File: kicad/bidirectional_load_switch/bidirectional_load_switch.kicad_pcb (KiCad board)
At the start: 2 copper layers, 0 parts

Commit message: load switch
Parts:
- added C101: 100n, Capacitor_SMD:C_0603_1608Metric, F.Cu at (133.9, 45.6)
- added C102: 10u, Capacitor_SMD:C_1206_3216Metric, F.Cu at (136.1, 45.6)
- added C103: 10u, Capacitor_SMD:C_1206_3216Metric, F.Cu at (127.0, 45.6)
- added C104: 100n, Capacitor_SMD:C_0603_1608Metric, F.Cu at (129.2, 45.6)
- added C201: 1u, Capacitor_SMD:C_0603_1608Metric, F.Cu at (126.4, 51.0)
- added C202: 100n, Capacitor_SMD:C_0603_1608Metric, F.Cu at (128.2, 51.0)
- added C203: 10u, Capacitor_SMD:C_1206_3216Metric, F.Cu at (150.1, 46.0)
- added C204: 100n, Capacitor_SMD:C_0603_1608Metric, F.Cu at (149.8, 48.0)
- added C301: 1u, Capacitor_SMD:C_0603_1608Metric, F.Cu at (126.4, 65.5)
- added C302: 100n, Capacitor_SMD:C_0603_1608Metric, F.Cu at (128.2, 65.5)
- added C303: 10u, Capacitor_SMD:C_1206_3216Metric, F.Cu at (150.1, 60.5)
- added C304: 100n, Capacitor_SMD:C_0603_1608Metric, F.Cu at (149.8, 62.5)
- added C401: 1u, Capacitor_SMD:C_0603_1608Metric, F.Cu at (126.4, 80.0)
- added C402: 100n, Capacitor_SMD:C_0603_1608Metric, F.Cu at (128.2, 80.0)
- added C403: 10u, Capacitor_SMD:C_1206_3216Metric, F.Cu at (150.1, 75.0)
- added C404: 100n, Capacitor_SMD:C_0603_1608Metric, F.Cu at (149.8, 77.0)
- added C501: 1u, Capacitor_SMD:C_0603_1608Metric, F.Cu at (126.4, 94.5)
- added C502: 100n, Capacitor_SMD:C_0603_1608Metric, F.Cu at (128.2, 94.5)
- added C503: 10u, Capacitor_SMD:C_1206_3216Metric, F.Cu at (150.1, 89.5)
- added C504: 100n, Capacitor_SMD:C_0603_1608Metric, F.Cu at (149.8, 91.5)
- added C601: 1u, Capacitor_SMD:C_0603_1608Metric, F.Cu at (126.4, 109.0)
- added C602: 100n, Capacitor_SMD:C_0603_1608Metric, F.Cu at (128.2, 109.0)
- added C603: 10u, Capacitor_SMD:C_1206_3216Metric, F.Cu at (150.1, 104.0)
- added C604: 100n, Capacitor_SMD:C_0603_1608Metric, F.Cu at (149.8, 106.0)
- added C701: 1u, Capacitor_SMD:C_0603_1608Metric, F.Cu at (126.4, 123.5)
- added C702: 100n, Capacitor_SMD:C_0603_1608Metric, F.Cu at (128.2, 123.5)
- added C703: 10u, Capacitor_SMD:C_1206_3216Metric, F.Cu at (150.1, 118.5)
- added C704: 100n, Capacitor_SMD:C_0603_1608Metric, F.Cu at (149.8, 120.5)
- added C801: 1u, Capacitor_SMD:C_0603_1608Metric, F.Cu at (126.4, 137.9)
- added C802: 100n, Capacitor_SMD:C_0603_1608Metric, F.Cu at (128.2, 137.9)
- added C803: 10u, Capacitor_SMD:C_1206_3216Metric, F.Cu at (150.1, 133.1)
- added C804: 100n, Capacitor_SMD:C_0603_1608Metric, F.Cu at (149.8, 135.1)
- added C901: 1u, Capacitor_SMD:C_0603_1608Metric, F.Cu at (126.4, 152.4)
- added C902: 100n, Capacitor_SMD:C_0603_1608Metric, F.Cu at (128.2, 152.4)
- added C903: 10u, Capacitor_SMD:C_1206_3216Metric, F.Cu at (150.1, 147.6)
- added C904: 100n, Capacitor_SMD:C_0603_1608Metric, F.Cu at (149.8, 149.6)
- added J101: 282838-2, screw_terminal_282838-2:CONN2_282838-2_TEC, F.Cu at (168.6, 38.1)
- added J102: Conn_01x02_Socket, Connector_PinHeader_2.54mm:PinHeader_1x02_P2.54mm_Vertical, F.Cu at (148.3, 41.1)
- added J103: Conn_01x09_Socket, Connector_PinHeader_2.54mm:PinHeader_1x09_P2.54mm_Vertical, F.Cu at (120.3, 41.1)
- added J104: Conn_01x02_Socket, Connector_PinHeader_2.54mm:PinHeader_1x02_P2.54mm_Vertical, F.Cu at (133.3, 41.1)
- added LED201: B1911PG--20D000514U1930, led_B1911PG--20D000514U1930:LED_B1911PG--20D000514U1930_HVK, F.Cu at (128.8, 54.9)
- added LED301: B1911PG--20D000514U1930, led_B1911PG--20D000514U1930:LED_B1911PG--20D000514U1930_HVK, F.Cu at (128.9, 69.3)
- added LED401: B1911PG--20D000514U1930, led_B1911PG--20D000514U1930:LED_B1911PG--20D000514U1930_HVK, F.Cu at (128.8, 83.8)
- added LED501: B1911PG--20D000514U1930, led_B1911PG--20D000514U1930:LED_B1911PG--20D000514U1930_HVK, F.Cu at (128.8, 98.3)
- added LED601: B1911PG--20D000514U1930, led_B1911PG--20D000514U1930:LED_B1911PG--20D000514U1930_HVK, F.Cu at (128.8, 112.8)
- added LED701: B1911PG--20D000514U1930, led_B1911PG--20D000514U1930:LED_B1911PG--20D000514U1930_HVK, F.Cu at (128.8, 127.3)
- added LED801: B1911PG--20D000514U1930, led_B1911PG--20D000514U1930:LED_B1911PG--20D000514U1930_HVK, F.Cu at (128.8, 141.8)
- added LED901: B1911PG--20D000514U1930, led_B1911PG--20D000514U1930:LED_B1911PG--20D000514U1930_HVK, F.Cu at (128.8, 156.3)
- added R201: 150, Resistor_SMD:R_0603_1608Metric, F.Cu at (131.8, 54.9)
- added R202: 50, Resistor_SMD:R_0603_1608Metric, F.Cu at (133.8, 49.9)
- added R203: 50, Resistor_SMD:R_0603_1608Metric, F.Cu at (133.8, 52.1)
- added R204: 5, Resistor_SMD:R_0805_2012Metric, F.Cu at (152.1, 50.0)
- added R205: 5, Resistor_SMD:R_0805_2012Metric, F.Cu at (152.1, 52.0)
- added R301: 150, Resistor_SMD:R_0603_1608Metric, F.Cu at (131.8, 69.3)
- added R302: 50, Resistor_SMD:R_0603_1608Metric, F.Cu at (133.8, 64.4)
- added R303: 50, Resistor_SMD:R_0603_1608Metric, F.Cu at (133.8, 66.6)
- added R304: 5, Resistor_SMD:R_0805_2012Metric, F.Cu at (152.1, 64.5)
- added R305: 5, Resistor_SMD:R_0805_2012Metric, F.Cu at (152.1, 66.5)
- added R401: 150, Resistor_SMD:R_0603_1608Metric, F.Cu at (131.8, 83.8)
- added R402: 50, Resistor_SMD:R_0603_1608Metric, F.Cu at (133.8, 78.9)
- added R403: 50, Resistor_SMD:R_0603_1608Metric, F.Cu at (133.8, 81.1)
- added R404: 5, Resistor_SMD:R_0805_2012Metric, F.Cu at (152.1, 79.0)
- added R405: 5, Resistor_SMD:R_0805_2012Metric, F.Cu at (152.1, 81.0)
- added R501: 150, Resistor_SMD:R_0603_1608Metric, F.Cu at (131.8, 98.3)
- added R502: 50, Resistor_SMD:R_0603_1608Metric, F.Cu at (133.8, 93.4)
- added R503: 50, Resistor_SMD:R_0603_1608Metric, F.Cu at (133.8, 95.6)
- added R504: 5, Resistor_SMD:R_0805_2012Metric, F.Cu at (152.1, 93.5)
- added R505: 5, Resistor_SMD:R_0805_2012Metric, F.Cu at (152.1, 95.5)
- added R601: 150, Resistor_SMD:R_0603_1608Metric, F.Cu at (131.8, 112.8)
- added R602: 50, Resistor_SMD:R_0603_1608Metric, F.Cu at (133.8, 107.9)
- added R603: 50, Resistor_SMD:R_0603_1608Metric, F.Cu at (133.8, 110.1)
- added R604: 5, Resistor_SMD:R_0805_2012Metric, F.Cu at (152.1, 108.0)
- added R605: 5, Resistor_SMD:R_0805_2012Metric, F.Cu at (152.1, 110.0)
- added R701: 150, Resistor_SMD:R_0603_1608Metric, F.Cu at (131.8, 127.3)
- added R702: 50, Resistor_SMD:R_0603_1608Metric, F.Cu at (133.8, 122.4)
- added R703: 50, Resistor_SMD:R_0603_1608Metric, F.Cu at (133.8, 124.6)
- added R704: 5, Resistor_SMD:R_0805_2012Metric, F.Cu at (152.1, 122.5)
- added R705: 5, Resistor_SMD:R_0805_2012Metric, F.Cu at (152.1, 124.5)
- added R801: 150, Resistor_SMD:R_0603_1608Metric, F.Cu at (131.8, 141.8)
- added R802: 50, Resistor_SMD:R_0603_1608Metric, F.Cu at (133.8, 136.9)
- added R803: 50, Resistor_SMD:R_0603_1608Metric, F.Cu at (133.8, 139.1)
- added R804: 5, Resistor_SMD:R_0805_2012Metric, F.Cu at (152.1, 137.1)
- added R805: 5, Resistor_SMD:R_0805_2012Metric, F.Cu at (152.1, 139.1)
- added R901: 150, Resistor_SMD:R_0603_1608Metric, F.Cu at (131.8, 156.3)
- added R902: 50, Resistor_SMD:R_0603_1608Metric, F.Cu at (133.8, 151.4)
- added R903: 50, Resistor_SMD:R_0603_1608Metric, F.Cu at (133.8, 153.6)
- added R904: 5, Resistor_SMD:R_0805_2012Metric, F.Cu at (152.1, 151.6)
- added R905: 5, Resistor_SMD:R_0805_2012Metric, F.Cu at (152.1, 153.6)
- added RS101: R_US, Resistor_SMD:R_2512_6332Metric, F.Cu at (163.5, 48.2)
- added RS102: R_US, Resistor_SMD:R_2512_6332Metric, F.Cu at (163.6, 62.6)
- added RS103: R_US, Resistor_SMD:R_2512_6332Metric, F.Cu at (163.6, 77.2)
- added RS104: R_US, Resistor_SMD:R_2512_6332Metric, F.Cu at (163.6, 91.7)
- added RS105: R_US, Resistor_SMD:R_2512_6332Metric, F.Cu at (163.6, 106.2)
- added RS106: R_US, Resistor_SMD:R_2512_6332Metric, F.Cu at (163.6, 120.7)
- added RS107: R_US, Resistor_SMD:R_2512_6332Metric, F.Cu at (163.6, 135.2)
- added RS108: R_US, Resistor_SMD:R_2512_6332Metric, F.Cu at (163.6, 149.7)
- added U101: LDL212PV33R, ldo_LDL212PV33R:DFN_V33R_STM, F.Cu at (131.6, 45.6)
- added U201: SN74LVC1G17DCKR, buffer_SN74LVC1G17DCKR:DCK5, F.Cu at (130.6, 51.0)
- added U202: UCC23313DWYR, gate_driver_UCC23313DWYR:SOIC6_DWY_TEX, F.Cu at (142.1, 51.0)
- added U203: SISS94DN-T1-GE3, mosfet_SISS94DN-T1-GE3:MOSFET_3DN-T1-GE3_VIS, F.Cu at (156.2, 48.7)
- added U204: SISS94DN-T1-GE3, mosfet_SISS94DN-T1-GE3:MOSFET_3DN-T1-GE3_VIS, F.Cu at (156.2, 54.4)
- added U301: SN74LVC1G17DCKR, buffer_SN74LVC1G17DCKR:DCK5, F.Cu at (130.6, 65.5)
- added U302: UCC23313DWYR, gate_driver_UCC23313DWYR:SOIC6_DWY_TEX, F.Cu at (142.1, 65.5)
- added U303: SISS94DN-T1-GE3, mosfet_SISS94DN-T1-GE3:MOSFET_3DN-T1-GE3_VIS, F.Cu at (156.2, 63.2)
- added U304: SISS94DN-T1-GE3, mosfet_SISS94DN-T1-GE3:MOSFET_3DN-T1-GE3_VIS, F.Cu at (156.2, 68.9)
- added U401: SN74LVC1G17DCKR, buffer_SN74LVC1G17DCKR:DCK5, F.Cu at (130.6, 80.0)
- added U402: UCC23313DWYR, gate_driver_UCC23313DWYR:SOIC6_DWY_TEX, F.Cu at (142.1, 80.0)
- added U403: SISS94DN-T1-GE3, mosfet_SISS94DN-T1-GE3:MOSFET_3DN-T1-GE3_VIS, F.Cu at (156.2, 77.7)
- added U404: SISS94DN-T1-GE3, mosfet_SISS94DN-T1-GE3:MOSFET_3DN-T1-GE3_VIS, F.Cu at (156.2, 83.4)
- added U501: SN74LVC1G17DCKR, buffer_SN74LVC1G17DCKR:DCK5, F.Cu at (130.6, 94.5)
- added U502: UCC23313DWYR, gate_driver_UCC23313DWYR:SOIC6_DWY_TEX, F.Cu at (142.1, 94.5)
- added U503: SISS94DN-T1-GE3, mosfet_SISS94DN-T1-GE3:MOSFET_3DN-T1-GE3_VIS, F.Cu at (156.2, 92.2)
- added U504: SISS94DN-T1-GE3, mosfet_SISS94DN-T1-GE3:MOSFET_3DN-T1-GE3_VIS, F.Cu at (156.2, 97.9)
- added U601: SN74LVC1G17DCKR, buffer_SN74LVC1G17DCKR:DCK5, F.Cu at (130.6, 109.0)
- added U602: UCC23313DWYR, gate_driver_UCC23313DWYR:SOIC6_DWY_TEX, F.Cu at (142.1, 109.0)
- added U603: SISS94DN-T1-GE3, mosfet_SISS94DN-T1-GE3:MOSFET_3DN-T1-GE3_VIS, F.Cu at (156.2, 106.7)
- added U604: SISS94DN-T1-GE3, mosfet_SISS94DN-T1-GE3:MOSFET_3DN-T1-GE3_VIS, F.Cu at (156.2, 112.4)
- added U701: SN74LVC1G17DCKR, buffer_SN74LVC1G17DCKR:DCK5, F.Cu at (130.6, 123.5)
- added U702: UCC23313DWYR, gate_driver_UCC23313DWYR:SOIC6_DWY_TEX, F.Cu at (142.1, 123.5)
- added U703: SISS94DN-T1-GE3, mosfet_SISS94DN-T1-GE3:MOSFET_3DN-T1-GE3_VIS, F.Cu at (156.2, 121.2)
- added U704: SISS94DN-T1-GE3, mosfet_SISS94DN-T1-GE3:MOSFET_3DN-T1-GE3_VIS, F.Cu at (156.2, 126.9)
- added U801: SN74LVC1G17DCKR, buffer_SN74LVC1G17DCKR:DCK5, F.Cu at (130.6, 138.0)
- added U802: UCC23313DWYR, gate_driver_UCC23313DWYR:SOIC6_DWY_TEX, F.Cu at (142.1, 138.0)
- added U803: SISS94DN-T1-GE3, mosfet_SISS94DN-T1-GE3:MOSFET_3DN-T1-GE3_VIS, F.Cu at (156.2, 135.7)
- added U804: SISS94DN-T1-GE3, mosfet_SISS94DN-T1-GE3:MOSFET_3DN-T1-GE3_VIS, F.Cu at (156.2, 141.4)
- added U901: SN74LVC1G17DCKR, buffer_SN74LVC1G17DCKR:DCK5, F.Cu at (130.6, 152.5)
- added U902: UCC23313DWYR, gate_driver_UCC23313DWYR:SOIC6_DWY_TEX, F.Cu at (142.1, 152.5)
- added U903: SISS94DN-T1-GE3, mosfet_SISS94DN-T1-GE3:MOSFET_3DN-T1-GE3_VIS, F.Cu at (156.2, 150.2)
- added U904: SISS94DN-T1-GE3, mosfet_SISS94DN-T1-GE3:MOSFET_3DN-T1-GE3_VIS, F.Cu at (156.2, 155.9)
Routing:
- net 3V3: track 0.00 -> 209.9 mm
- net /PWM8: track 0.00 -> 106.1 mm
- net /PWM7: track 0.00 -> 94.1 mm
- net /PWM6: track 0.00 -> 82.1 mm
- net /PWM5: track 0.00 -> 70.1 mm
- net /PWM4: track 0.00 -> 58.2 mm
- net /PWM3: track 0.00 -> 46.1 mm
- net /PWM2: track 0.00 -> 34.2 mm
- net /PWM1: track 0.00 -> 22.3 mm
- net GND: track 0.00 -> 10.5 mm, vias 0 -> 78
- net Net-(U902-CATHODE): track 0.00 -> 2.15 mm
- net Net-(U802-CATHODE): track 0.00 -> 2.15 mm
- net Net-(U702-CATHODE): track 0.00 -> 2.15 mm
- net Net-(U602-CATHODE): track 0.00 -> 2.15 mm
- net Net-(U502-CATHODE): track 0.00 -> 2.15 mm
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- added copper zone on F.Cu, net /AC_in
- added copper zone on F.Cu, net /Channel 1/RIN
- added copper zone on F.Cu, net /Channel 2/RIN
- added copper zone on F.Cu, net /Channel 3/RIN
- added copper zone on F.Cu, net /Channel 4/RIN
- added copper zone on F.Cu, net /Channel 5/RIN
- added copper zone on F.Cu, net /Channel 6/RIN
- added copper zone on F.Cu, net /Channel 7/RIN
- added copper zone on F.Cu, net /Channel 8/RIN
- added copper zone on B.Cu, net 15V_isolated
- added copper zone on F.Cu, net 15V_isolated
- added copper zone on F.Cu, net 3V3
- added copper zone on F.Cu, net 5V
- added copper zone on B.Cu, net Earth
- added copper zone on F.Cu, net Earth
- added copper zone on B.Cu, net GND
- added copper zone on F.Cu, net GND
- added copper zone on B.Cu, net GNDPWR
- added copper zone on F.Cu, net GNDPWR
- added copper zone on F.Cu, net Net-(U202-VOUT)
- added copper zone on F.Cu, net Net-(U203-G)
- added copper zone on F.Cu, net Net-(U204-G)
- added copper zone on F.Cu, net Net-(U302-VOUT)
- added copper zone on F.Cu, net Net-(U303-G)
- added copper zone on F.Cu, net Net-(U304-G)
- added copper zone on F.Cu, net Net-(U402-VOUT)
- added copper zone on F.Cu, net Net-(U403-G)
- added copper zone on F.Cu, net Net-(U404-G)
- added copper zone on F.Cu, net Net-(U502-VOUT)
- added copper zone on F.Cu, net Net-(U503-G)
- added copper zone on F.Cu, net Net-(U504-G)
- added copper zone on F.Cu, net Net-(U602-VOUT)
- added copper zone on F.Cu, net Net-(U603-G)
- added copper zone on F.Cu, net Net-(U604-G)
- added copper zone on F.Cu, net Net-(U702-VOUT)
- added copper zone on F.Cu, net Net-(U703-G)
- added copper zone on F.Cu, net Net-(U704-G)
- added copper zone on F.Cu, net Net-(U802-VOUT)
- added copper zone on F.Cu, net Net-(U803-G)
- added copper zone on F.Cu, net Net-(U804-G)
- added copper zone on F.Cu, net Net-(U902-VOUT)
- added copper zone on F.Cu, net Net-(U903-G)
- added copper zone on F.Cu, net Net-(U904-G)
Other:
- board outline added: 54.7 x 125.5 mm

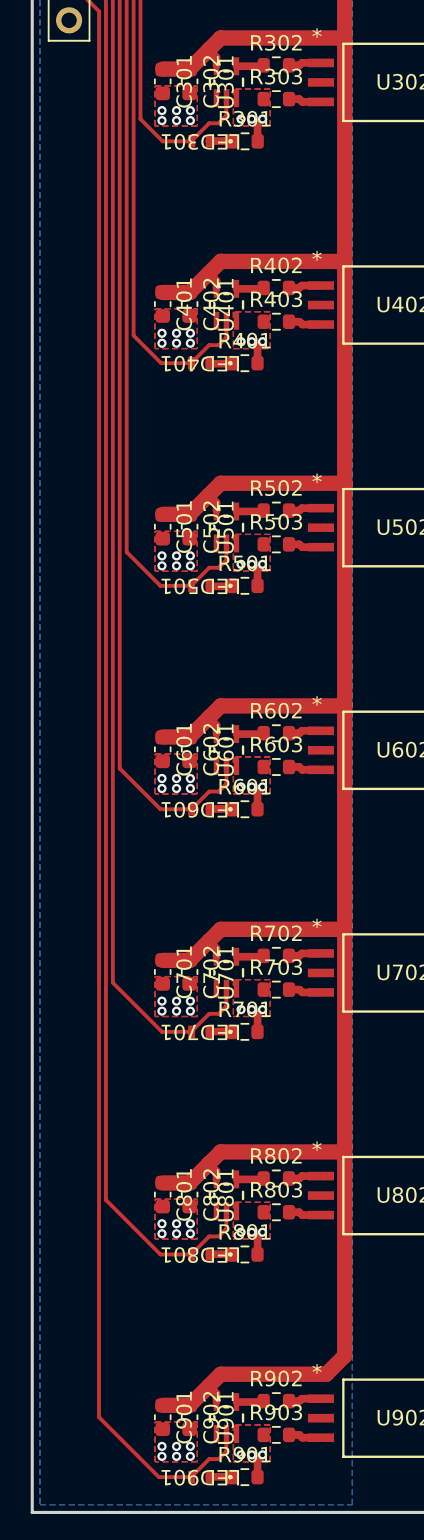
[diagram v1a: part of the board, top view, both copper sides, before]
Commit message: kicad
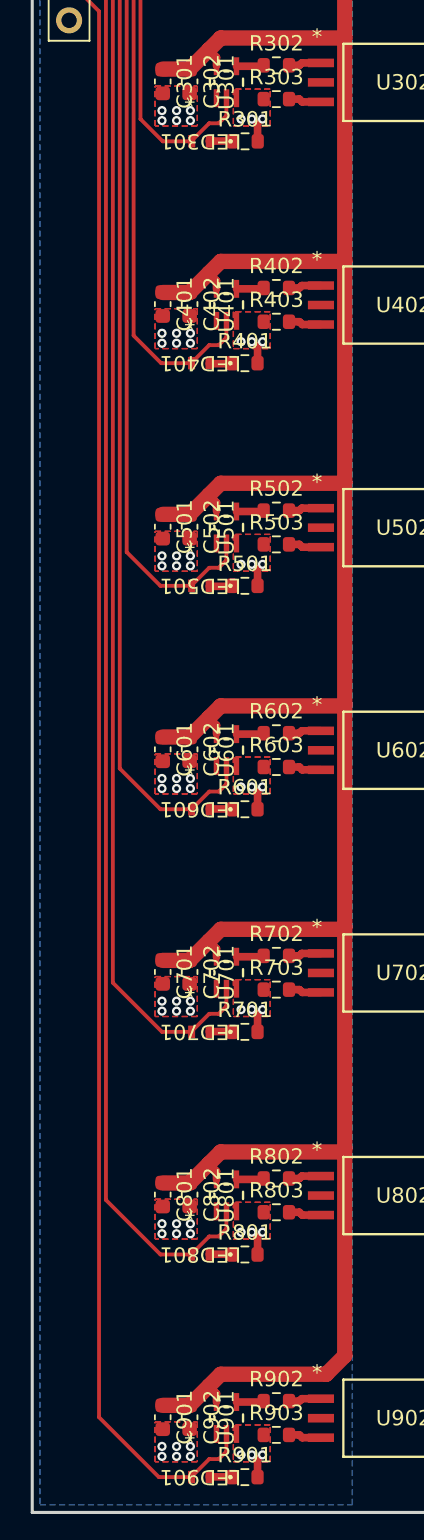
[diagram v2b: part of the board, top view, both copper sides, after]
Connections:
- net Net-(U201-Y) renamed /Channel 1/BOUT
- net Net-(U202-ANODE) renamed /Channel 1/ANODE
- net Net-(U202-VOUT) renamed /Channel 1/VOUT
- net Net-(U203-G) renamed /Channel 1/VG1
- net Net-(U204-G) renamed /Channel 1/VG2
- net Net-(U301-Y) renamed /Channel 2/BOUT
- net Net-(U302-ANODE) renamed /Channel 2/ANODE
- net Net-(U302-VOUT) renamed /Channel 2/VOUT
- net Net-(U303-G) renamed /Channel 2/VG1
- net Net-(U304-G) renamed /Channel 2/VG2
- net Net-(U401-Y) renamed /Channel 3/BOUT
- net Net-(U402-ANODE) renamed /Channel 3/ANODE
- net Net-(U402-VOUT) renamed /Channel 3/VOUT
- net Net-(U403-G) renamed /Channel 3/VG1
- net Net-(U404-G) renamed /Channel 3/VG2
- net Net-(U501-Y) renamed /Channel 4/BOUT
- net Net-(U502-ANODE) renamed /Channel 4/ANODE
- net Net-(U502-VOUT) renamed /Channel 4/VOUT
- net Net-(U503-G) renamed /Channel 4/VG1
- net Net-(U504-G) renamed /Channel 4/VG2
- net Net-(U601-Y) renamed /Channel 5/BOUT
- net Net-(U602-ANODE) renamed /Channel 5/ANODE
- net Net-(U602-VOUT) renamed /Channel 5/VOUT
- net Net-(U603-G) renamed /Channel 5/VG1
- net Net-(U604-G) renamed /Channel 5/VG2
- net Net-(U701-Y) renamed /Channel 6/BOUT
- net Net-(U702-ANODE) renamed /Channel 6/ANODE
- net Net-(U702-VOUT) renamed /Channel 6/VOUT
- net Net-(U703-G) renamed /Channel 6/VG1
- net Net-(U704-G) renamed /Channel 6/VG2
- net Net-(U801-Y) renamed /Channel 7/BOUT
- net Net-(U802-ANODE) renamed /Channel 7/ANODE
- net Net-(U802-VOUT) renamed /Channel 7/VOUT
- net Net-(U803-G) renamed /Channel 7/VG1
- net Net-(U804-G) renamed /Channel 7/VG2
- net Net-(U901-Y) renamed /Channel 8/BOUT
- net Net-(U902-ANODE) renamed /Channel 8/ANODE
- net Net-(U902-VOUT) renamed /Channel 8/VOUT
- net Net-(U903-G) renamed /Channel 8/VG1
- net Net-(U904-G) renamed /Channel 8/VG2

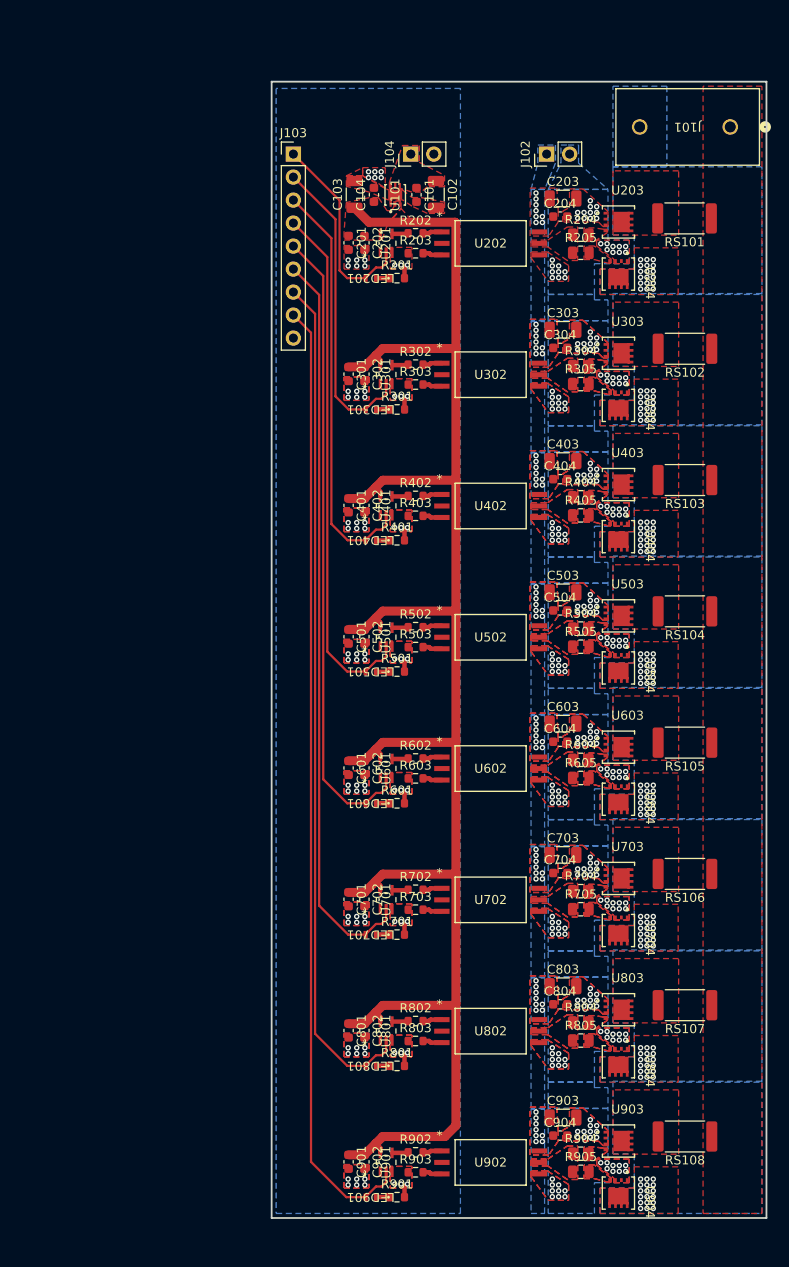
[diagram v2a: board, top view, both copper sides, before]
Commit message: kicad
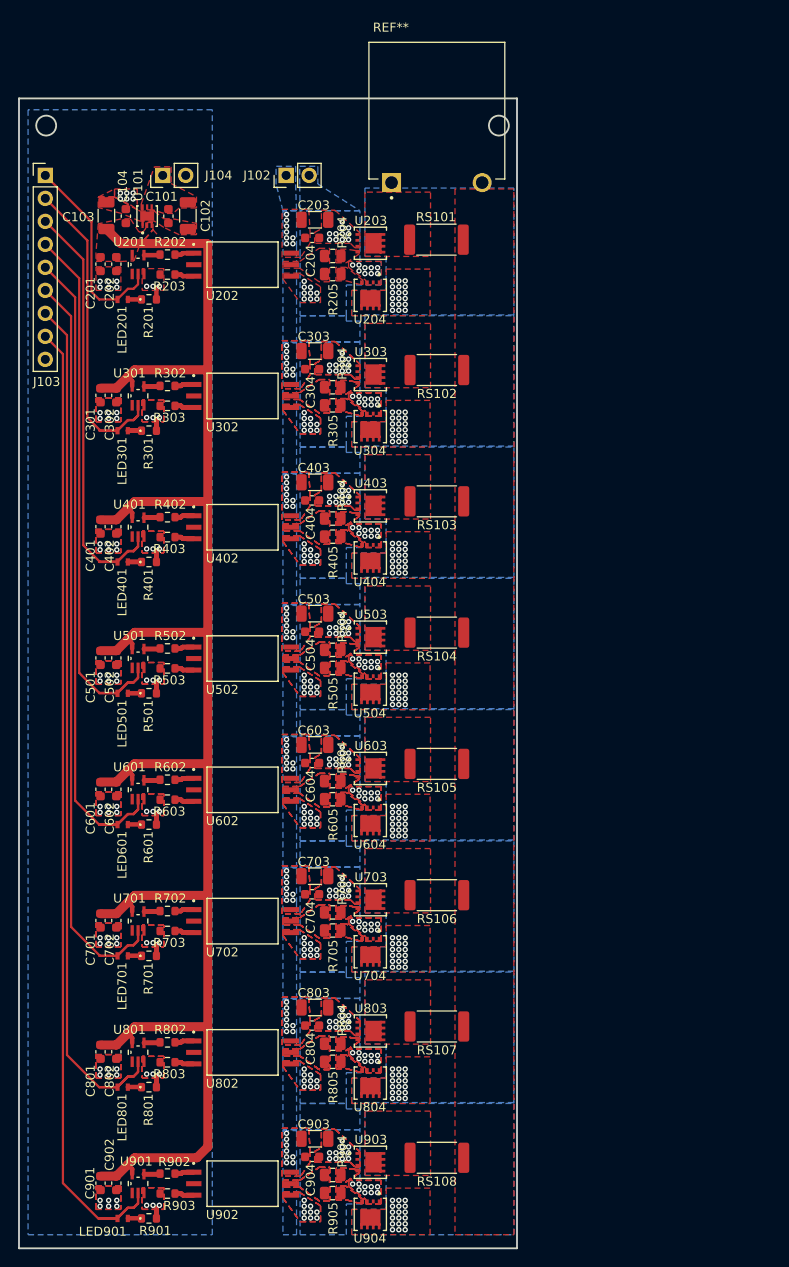
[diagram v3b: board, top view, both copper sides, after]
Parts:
- removed J101: 282838-2, screw_terminal_282838-2:CONN2_282838-2_TEC
- added REF**: TE_282852-2, screw_terminal_282852-2:TE_282852-2, F.Cu at (136.2, 44.3)
- RS101: value R_US -> 1
- RS102: value R_US -> 3.9
- RS103: value R_US -> 15
- RS104: value R_US -> 47
- RS105: value R_US -> 200
- RS106: value R_US -> 680
- RS107: value R_US -> 2700
- RS108: value R_US -> 10000
- moved J102 28.9 mm to (119.5, 43.5)
- moved R301 27.5 mm to (104.3, 71.7)
- moved LED301 27.5 mm to (101.5, 71.7)
- moved R401 27.5 mm to (104.3, 86.2)
- moved R501 27.5 mm to (104.3, 100.7)
- moved LED501 27.5 mm to (101.5, 100.7)
- moved LED401 27.5 mm to (101.5, 86.2)
- moved C101 27.5 mm to (106.5, 48.0)
- moved C102 27.5 mm to (108.7, 48.0)
- moved C201 27.5 mm to (99.0, 53.3)
- moved C202 27.5 mm to (100.8, 53.3)
- moved C204 27.5 mm to (122.4, 50.4)
- moved C301 27.5 mm to (99.0, 67.8)
- moved C302 27.5 mm to (100.8, 67.8)
- moved C304 27.5 mm to (122.4, 64.9)
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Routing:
- net GND: track 10.5 -> 18.6 mm
- net /PWM8: track 106.1 -> 112.3 mm
- net /PWM7: track 94.1 -> 100.3 mm
- net /PWM2: track 34.2 -> 40.4 mm
- net /PWM6: track 82.1 -> 88.3 mm
- net /PWM5: track 70.1 -> 76.3 mm
- net /PWM4: track 58.2 -> 64.4 mm
- net /PWM3: track 46.1 -> 52.3 mm
- net Net-(U902-CATHODE): track 2.15 -> 4.31 mm
- net Net-(U802-CATHODE): track 2.15 -> 4.31 mm
- net Net-(U502-CATHODE): track 2.15 -> 4.31 mm
- net Net-(U702-CATHODE): track 2.15 -> 4.31 mm
- net Net-(U602-CATHODE): track 2.15 -> 4.31 mm
- net Net-(U402-CATHODE): track 2.15 -> 4.31 mm
- net Net-(U302-CATHODE): track 2.15 -> 4.31 mm
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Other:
- board size 54.7 x 125.5 mm -> 55 x 127 mm
- board text added: "0.1524 mm / 0.1524 mm"
- board text added: "0.2540 mm"
- board text added: "1.6000 mm"
- board text added: "2"
- board text added: "55.6500 mm x 126.5000 mm"
- board text added: "BOARD CHARACTERISTICS"
- board text added: "Board Thickness:"
- board text added: "Board overall dimensions:"
- board text added: "Castellated pads:"
- board text added: "Copper Finish:"
- board text added: "Copper Layer Count:"
- board text added: "ENIG"
- board text added: "Edge card connectors:"
- board text added: "Impedance Control:"
- board text added: "Min hole diameter:"
- board text added: "Min track/spacing:"
- board text added: "No"
- board text added: "Plated Board Edge:"
